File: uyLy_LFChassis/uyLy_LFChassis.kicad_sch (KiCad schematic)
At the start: 9 parts, among them J1 Conn_01x08_Socket, J2 Conn_01x02_Pin, J3 Conn_01x02_Pin, J4 Conn_01x02_Pin, J5 Conn_01x02_Socket, J6 Conn_01x01_Socket, SW1 SW_DIP_x04, U1 TB6612FNG

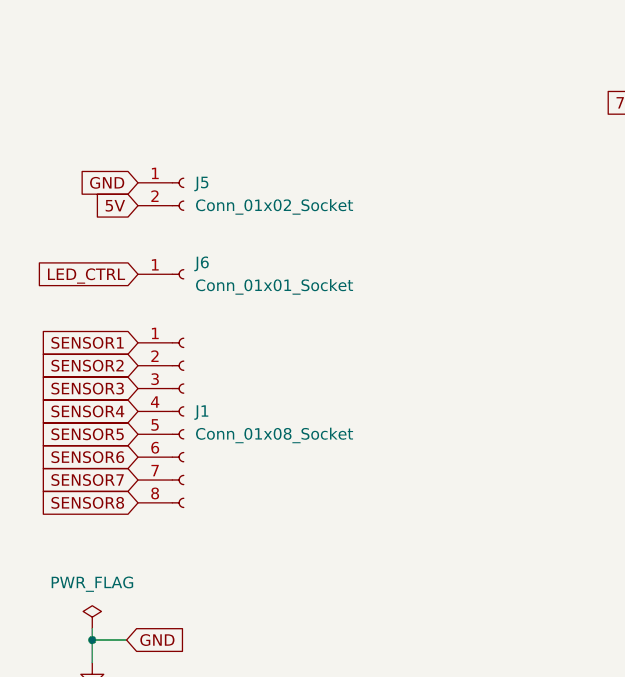
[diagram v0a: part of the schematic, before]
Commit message: update: pcb design
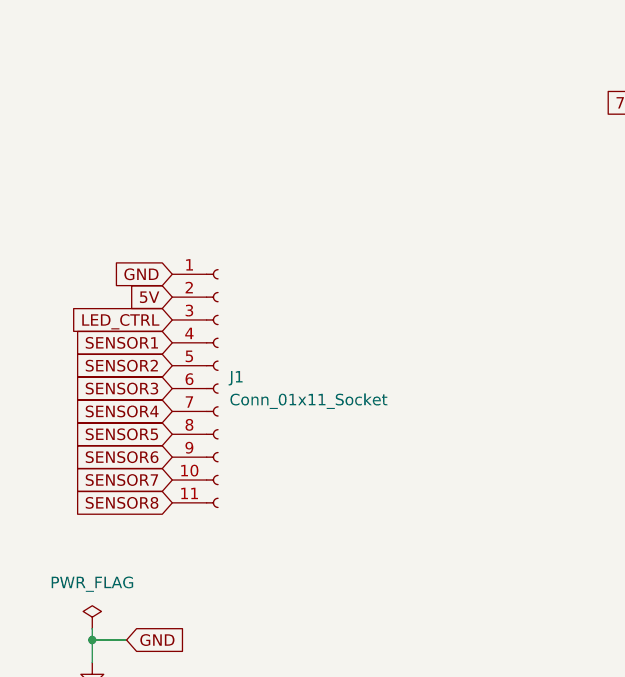
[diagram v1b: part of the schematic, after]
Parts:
- removed J1: Conn_01x08_Socket, Connector_PinHeader_2.54mm:PinHeader_1x08_P2.54mm_Vertical, symbol Connector:Conn_01x08_Socket
- removed J5: Conn_01x02_Socket, Connector_PinHeader_2.54mm:PinHeader_1x02_P2.54mm_Horizontal, symbol Connector:Conn_01x02_Socket
- removed J6: Conn_01x01_Socket, Connector_PinHeader_2.54mm:PinHeader_1x01_P2.54mm_Horizontal, symbol Connector:Conn_01x01_Socket
- added J1: Conn_01x11_Socket, Connector_PinHeader_2.54mm:PinHeader_1x11_P2.54mm_Vertical, symbol Connector:Conn_01x11_Socket
- J4: footprint Connector_JST:JST_XH_S2B-XH-A_1x02_P2.50mm_Horizontal -> Connector_JST:JST_XH_B2B-XH-A_1x02_P2.50mm_Vertical
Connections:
- net 5V: now also J1.2 (Pin_2)
- net GND: now also J1.1 (Pin_1)
- net LED_CTRL: now also J1.3 (Pin_3)
- net SENSOR1: now also J1.4 (Pin_4)
- net SENSOR2: now also J1.5 (Pin_5)
- net SENSOR3: now also J1.6 (Pin_6)
- net SENSOR4: now also J1.7 (Pin_7)
- net SENSOR5: now also J1.8 (Pin_8)
- net SENSOR6: now also J1.9 (Pin_9)
- net SENSOR7: now also J1.10 (Pin_10)
- net SENSOR8: now also J1.11 (Pin_11)
